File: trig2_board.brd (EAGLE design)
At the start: 80 x 123 mm, 33 parts, among them J1 2p-2.54, J13 8pin, J2 2p-2.54, J3 2p-2.54, J4 2p-2.54, J5 2p-2.54, J6 2p-2.54, J7 2p-2.54, J8 2p-2.54, X1 BU-SMB-V, X13 87758-2816, X14 87758-2816, X15 87758-1616, X16 87758-1616, X17 87758-2816, X18 87758-2816, X2 BU-SMB-V, X3 BU-SMB-V, X4 BU-SMB-V, X5 BU-SMB-V, X6 BU-SMB-V, X7 BU-SMB-V, X8 BU-SMB-V

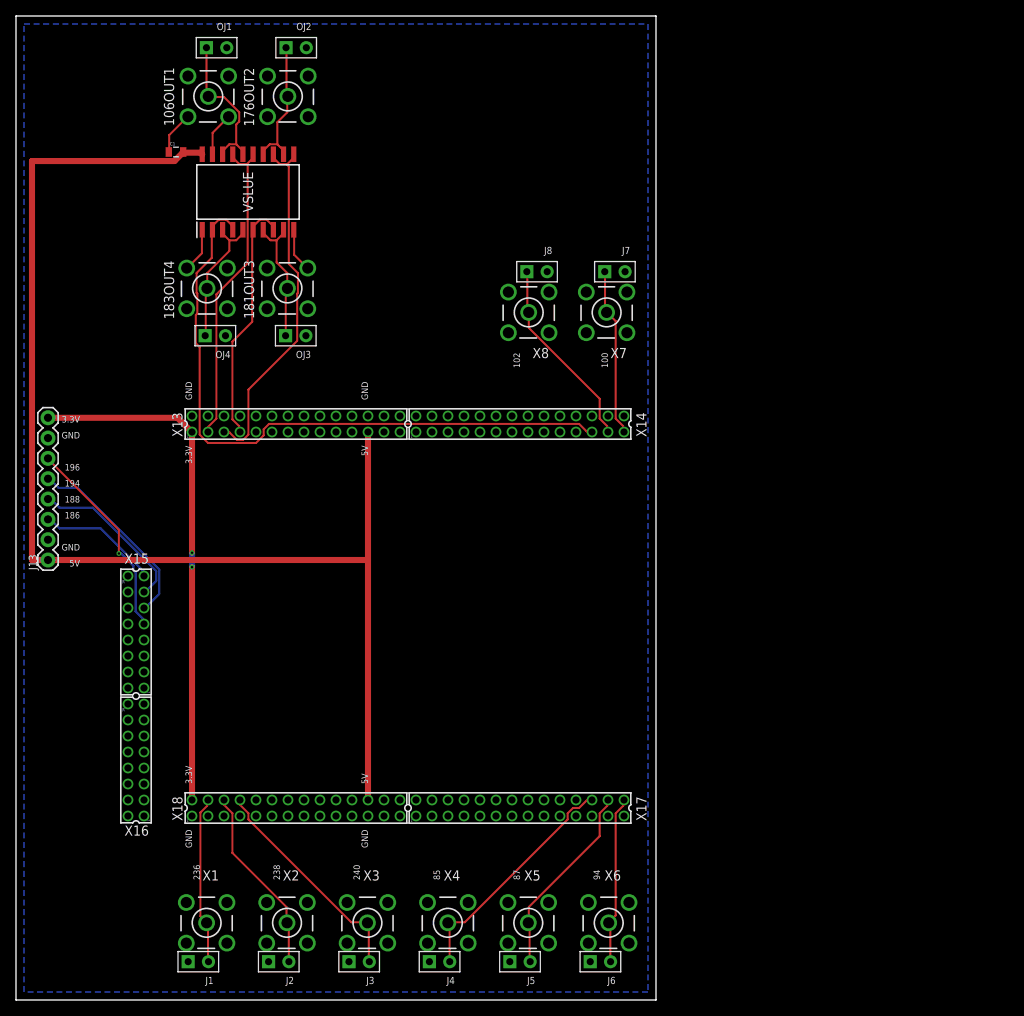
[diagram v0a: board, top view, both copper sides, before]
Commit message: with design block
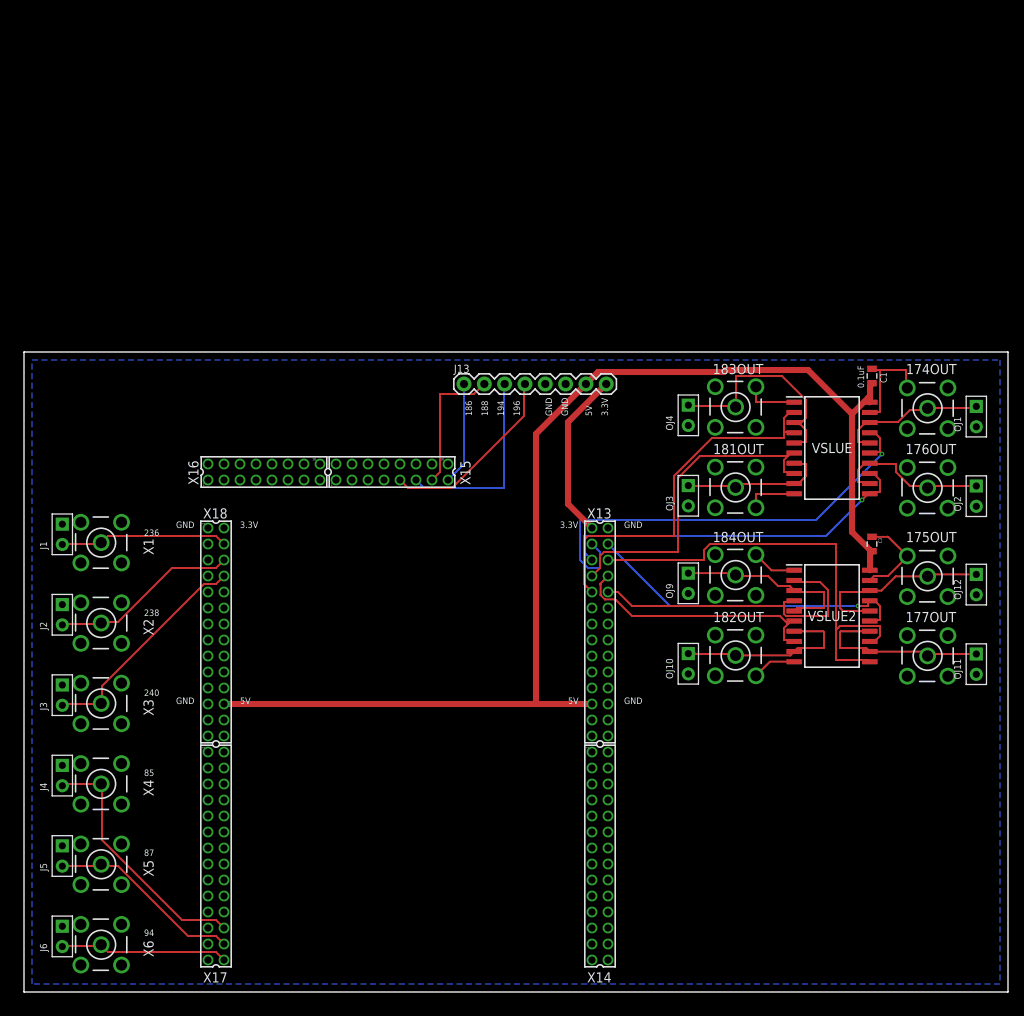
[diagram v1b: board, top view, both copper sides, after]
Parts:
- removed 106OUT1, 176OUT2, 181OUT3, 183OUT4, X7, X8: BU-SMB-V, con-coax:BU-SMB-V
- removed J7, J8: 2p-2.54, Seeed-Connector:H2-2.54
- added 174OUT, 175OUT, 176OUT, 177OUT, 181OUT, 182OUT, 183OUT, 184OUT: BU-SMB-V, con-coax:BU-SMB-V
- added C3: 0.1uF, SparkFun-Capacitors:0805
- added OJ10, OJ11, OJ12, OJ9: 2p-2.54, Seeed-Connector:H2-2.54
- added VSLUE2: SN74ACT244DW, SN74ACT244DW:SOIC127P1030X265-20N
- C1: value (none) -> 0.1uF
- moved OJ1 105.6 mm to (120.0, 72.9), turned to 0 degrees
- moved OJ2 101.8 mm to (120.0, 63.0), turned to 0 degrees
- moved C1 91.4 mm to (107.0, 78.0), turned to 270 degrees
- moved VSLUE 79.7 mm to (102.0, 69.0), turned to 0 degrees
- moved J6 67.3 mm to (5.79, 7.95), turned to 0 degrees
- moved X6 63.5 mm to (10.7, 6.91), turned to 90 degrees
- moved OJ4 60.0 mm to (84.0, 73.1), turned to 0 degrees
- moved J5 58.7 mm to (5.79, 18.0), turned to 0 degrees
- moved J13 56.5 mm to (56.0, 77.0), turned to 0 degrees
- moved J1 56.1 mm to (5.79, 58.2), turned to 0 degrees
- moved X14 54.9 mm to (73.0, 18.0), turned to 270 degrees
- moved X5 53.9 mm to (10.7, 17.0), turned to 90 degrees
- moved OJ3 53.0 mm to (84.0, 63.0), turned to 0 degrees
- moved J4 52.6 mm to (5.79, 28.1), turned to 0 degrees
- moved J2 51.1 mm to (5.79, 48.2), turned to 0 degrees
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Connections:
- removed net IO100: J7.1, X14.27, X7.1
- removed net IO102: J8.1, X14.25, X8.1
- removed net IO106_IN1: VSLUE.2, VSLUE.4, X14.23
- new net IO174_IN1: VSLUE.2, VSLUE.4, X13.9
- new net IO175_IN1: VSLUE2.2, VSLUE2.4, X13.10
- new net IO177_IN2: VSLUE2.6, VSLUE2.8, X13.8
- new net IO182_IN3: VSLUE2.11, VSLUE2.13, X13.6
- new net IO184_IN4: VSLUE2.15, VSLUE2.17, X13.4
- new net OUT5: 175OUT.1, OJ12.1, VSLUE2.16, VSLUE2.18
- new net OUT6: 177OUT.1, OJ11.1, VSLUE2.12, VSLUE2.14
- new net OUT7: 182OUT.1, OJ10.1, VSLUE2.7, VSLUE2.9
- new net OUT8: 184OUT.1, OJ9.1, VSLUE2.3, VSLUE2.5
- net 3V3: no longer X18.2
- net 5V: now also C3.2, J13.7, VSLUE2.20; no longer J13.1
- net GND: now also 174OUT.2, 174OUT.3, 174OUT.4, 174OUT.5, 175OUT.2, 175OUT.3, 175OUT.4, 175OUT.5, 176OUT.2, 176OUT.3, 176OUT.4, 176OUT.5, 177OUT.2, 177OUT.3, 177OUT.4, 177OUT.5, 181OUT.2, 181OUT.3, 181OUT.4, 181OUT.5, 182OUT.2, 182OUT.3, 182OUT.4, 182OUT.5, 183OUT.2, 183OUT.3, 183OUT.4, 183OUT.5, 184OUT.2, 184OUT.3, 184OUT.4, 184OUT.5, C3.1, J13.5, J13.6, OJ10.2, OJ11.2, OJ12.2, OJ9.2, VSLUE2.1, VSLUE2.10, VSLUE2.19; no longer 106OUT1.2, 106OUT1.3, 106OUT1.4, 106OUT1.5, 176OUT2.2, 176OUT2.3, 176OUT2.4, 176OUT2.5, 181OUT3.2, 181OUT3.3, 181OUT3.4, 181OUT3.5, 183OUT4.2, 183OUT4.3, 183OUT4.4, 183OUT4.5, J13.2, J13.7, J7.2, J8.2, X7.2, X7.3, X7.4, X7.5, X8.2, X8.3, X8.4, X8.5
- net IO186: now also J13.1; no longer J13.3
- net IO188: now also J13.2; no longer J13.4
- net IO194: now also J13.3; no longer J13.5
- net IO196: now also J13.4; no longer J13.6
- net OUT1: now also 174OUT.1; no longer 106OUT1.1
- net OUT2: now also 176OUT.1; no longer 176OUT2.1
- net OUT3: now also 181OUT.1; no longer 181OUT3.1
- net OUT4: now also 183OUT.1; no longer 183OUT4.1
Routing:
- net IO106_IN1: track 82.2 -> 0.00 mm
- net IO182_IN3: track 0.00 -> 57.5 mm
- net IO174_IN1: track 0.00 -> 47.1 mm
- net 3V3: track 64.7 -> 21.2 mm, vias 2 -> 0
- net IO184_IN4: track 0.00 -> 41.2 mm, vias 0 -> 1
- net IO175_IN1: track 0.00 -> 39.2 mm
- net IO177_IN2: track 0.00 -> 32.4 mm
- net GND: track 22.1 -> 49.0 mm
- net IO102: track 24.3 -> 0.00 mm
- net OUT8: track 0.00 -> 23.8 mm
- net OUT5: track 0.00 -> 23.8 mm
- net OUT6: track 0.00 -> 23.3 mm
- net OUT7: track 0.00 -> 23.2 mm
- net IO100: track 21.1 -> 0.00 mm
- net IO183_IN4: track 39.7 -> 57.6 mm, vias 0 -> 1
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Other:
- board size 80 x 123 mm -> 123 x 80 mm
- board text removed: "100"
- board text removed: "102"
